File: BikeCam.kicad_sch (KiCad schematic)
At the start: 23 parts, among them IC1 FS312F-G, J1 USB_OTG, J2 Conn_01x02_Female, Q1 IRLZ34N, Q2 IRLZ34N, Q3 IRLML5203, Q4 IRLML5203, U1 MCP73831-2-OT, U2 LTC3531ES6-3_3

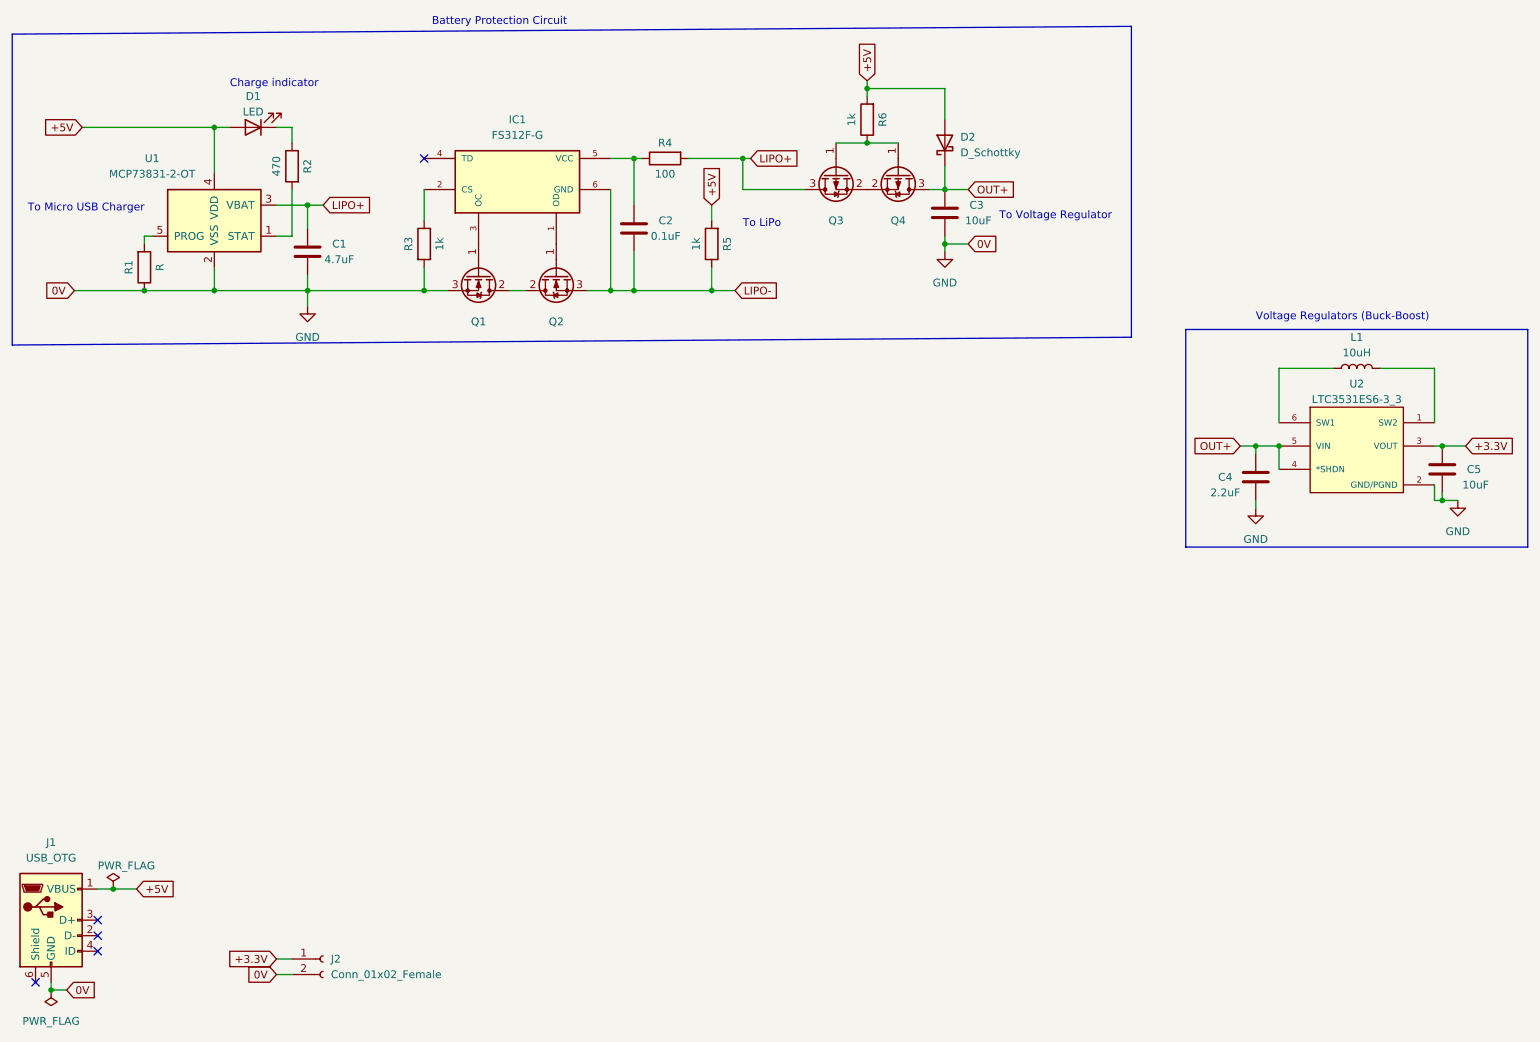
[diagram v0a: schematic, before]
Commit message: pcb trace
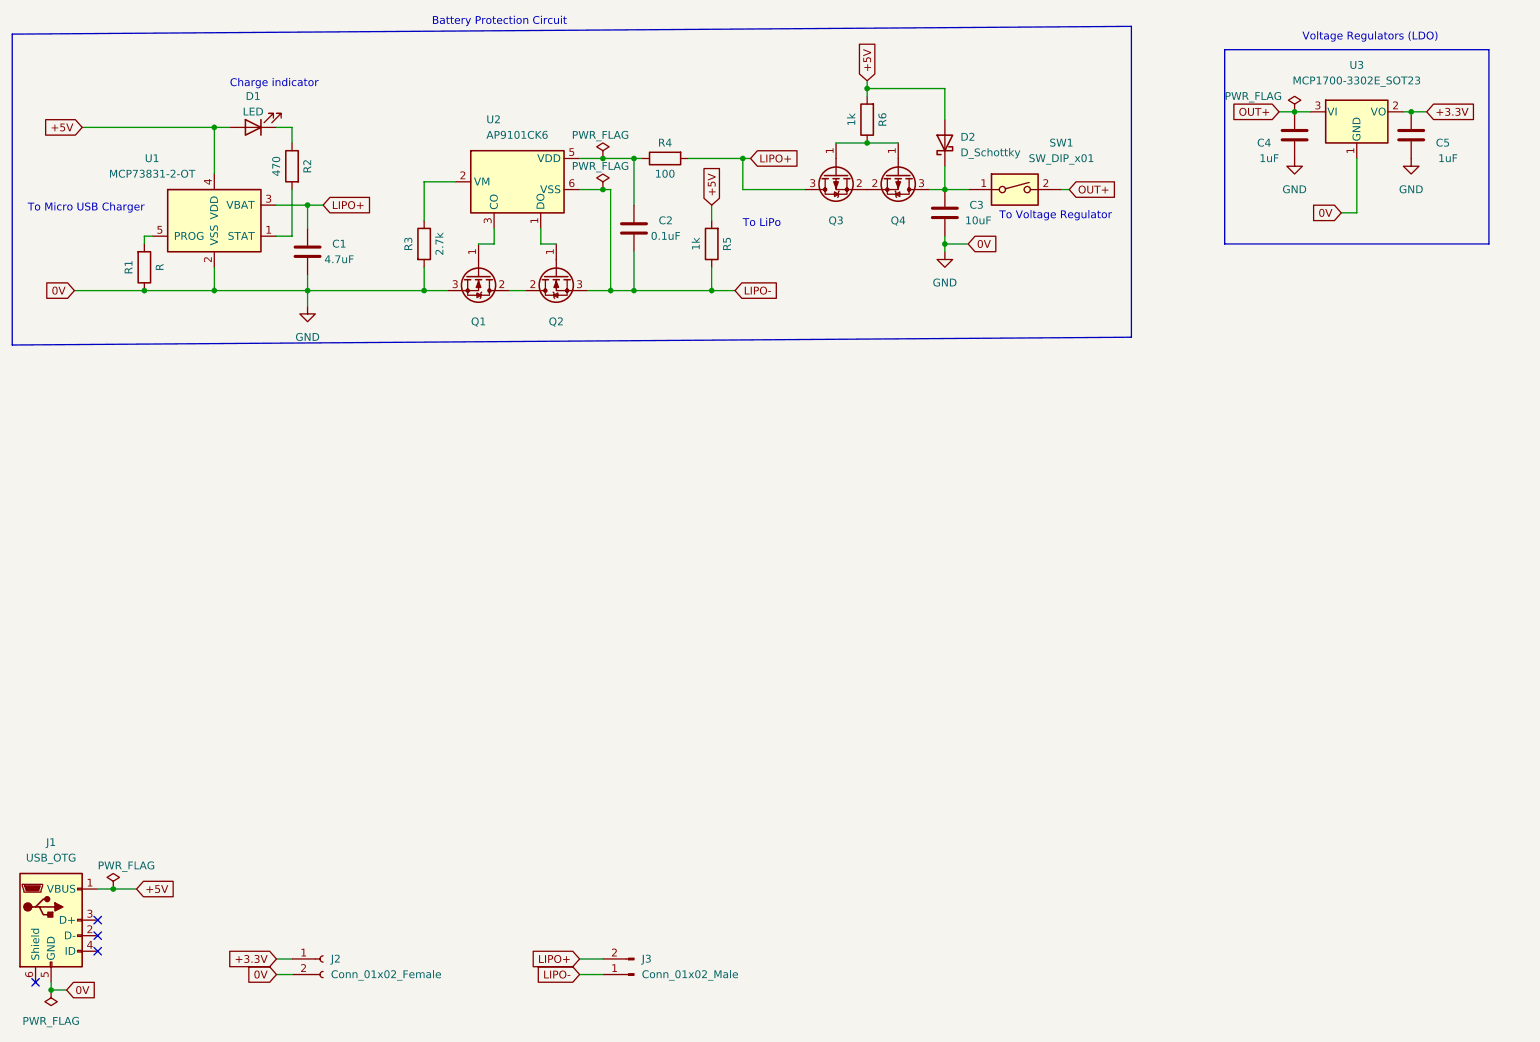
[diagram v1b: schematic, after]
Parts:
- removed IC1: FS312F-G, Package_TO_SOT_SMD:SOT-23-6, symbol FS312F-G:FS312F-G
- removed L1: 10uH, Inductor_SMD:L_1812_4532Metric, symbol Device:L
- removed U2: LTC3531ES6-3_3, Package_TO_SOT_SMD:TSOT-23-6, symbol LTC3531ES6-3_3:LTC3531ES6-3_3
- added J3: Conn_01x02_Male, Connector_PinHeader_1.00mm:PinHeader_1x02_P1.00mm_Vertical, symbol Connector:Conn_01x02_Male
- added SW1: SW_DIP_x01, Connector_PinHeader_1.00mm:PinHeader_1x02_P1.00mm_Vertical, symbol Switch:SW_DIP_x01
- added U2: AP9101CK6, Package_TO_SOT_SMD:SOT-23-6, symbol Battery_Management:AP9101CK6
- added U3: MCP1700-3302E_SOT23, Package_TO_SOT_SMD:SOT-23, symbol Regulator_Linear:MCP1700-3302E_SOT23
- C4: value 2.2uF -> 1uF
- C5: value 10uF -> 1uF
- R3: value 1k -> 2.7k
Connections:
- net +3.3V: now also U3.2 (VO)
- net GND: now also U3.1 (GND)
- net LIPO+: now also J3.2 (Pin_2)
- net LIPO-: now also J3.1 (Pin_1), U2.6 (VSS)
- net OUT+: now also SW1.2, U3.3 (VI); no longer C3.2, D2.1 (K), Q4.3 (D)
- net at C2.2, R4.1: now also U2.5 (VDD)
- net at Q2.1 (G): now also U2.1 (DO)
- net at R3.1: now also U2.2 (VM)
- net at Q1.1 (G): now also U2.3 (CO)
- new net: C3.2, D2.1 (K), Q4.3 (D), SW1.1
- no-connect marks 5 -> 4
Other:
- note added: "Voltage Regulators (LDO)"
- note removed: "Voltage Regulators (Buck-Boost)"
